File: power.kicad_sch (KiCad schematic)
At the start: 19 parts, among them J1 USB_B_Micro_Console, J4 USB_B_Micro_Power, U1 SRV05-4

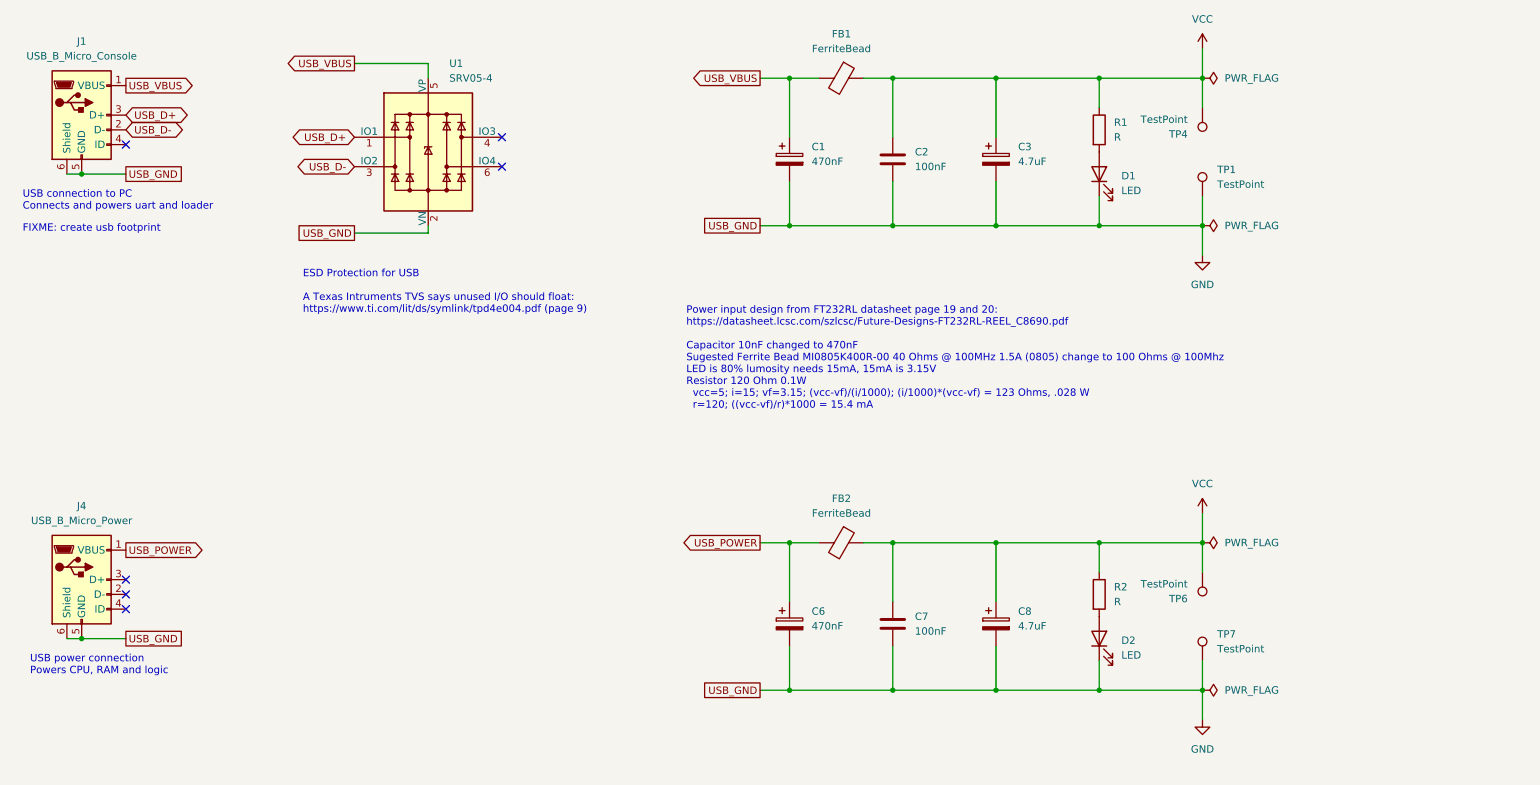
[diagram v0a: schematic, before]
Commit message: updates
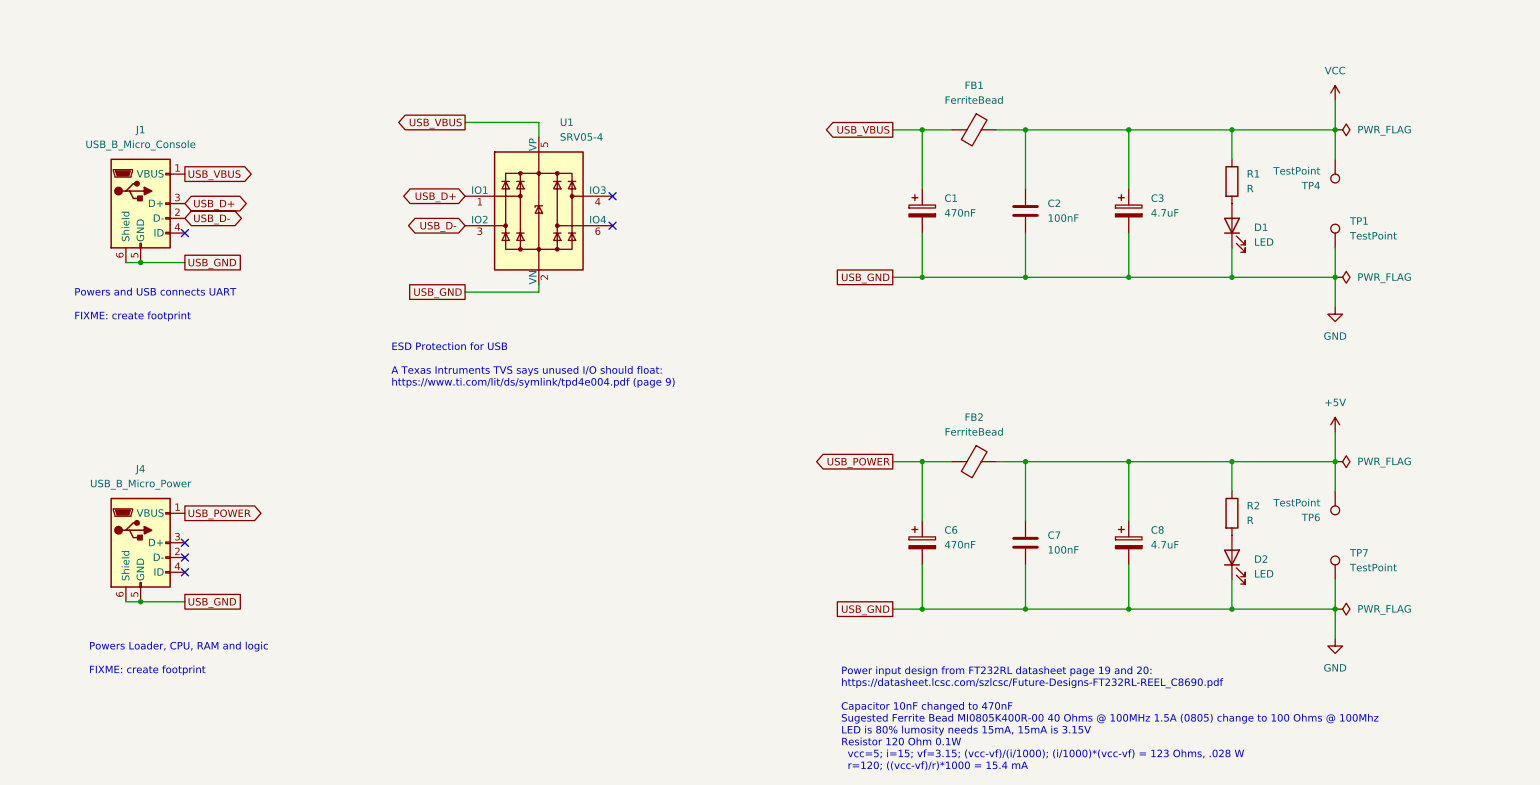
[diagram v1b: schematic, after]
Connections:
- net VCC: no longer C7.1, C8.1, FB2.1, R2.1, TP6.1
- new net +5V: C7.1, C8.1, FB2.1, R2.1, TP6.1
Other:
- note added: "Powers Loader, CPU, RAM and logic FIXME: create footprint"
- note added: "Powers and USB connects UART FIXME: create footprint"
- note removed: "FIXME: create usb footprint"
- note removed: "USB connection to PC Connects and powers uart and loader"
- note removed: "USB power connection Powers CPU, RAM and logic"
- moved on the sheet: C1, C2, C3, C6, C7, C8, D1, D2, FB1, FB2, J1, J4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
